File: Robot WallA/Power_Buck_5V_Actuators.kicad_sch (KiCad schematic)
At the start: 18 parts, among them J14 NID35-5, Q1 BSS138

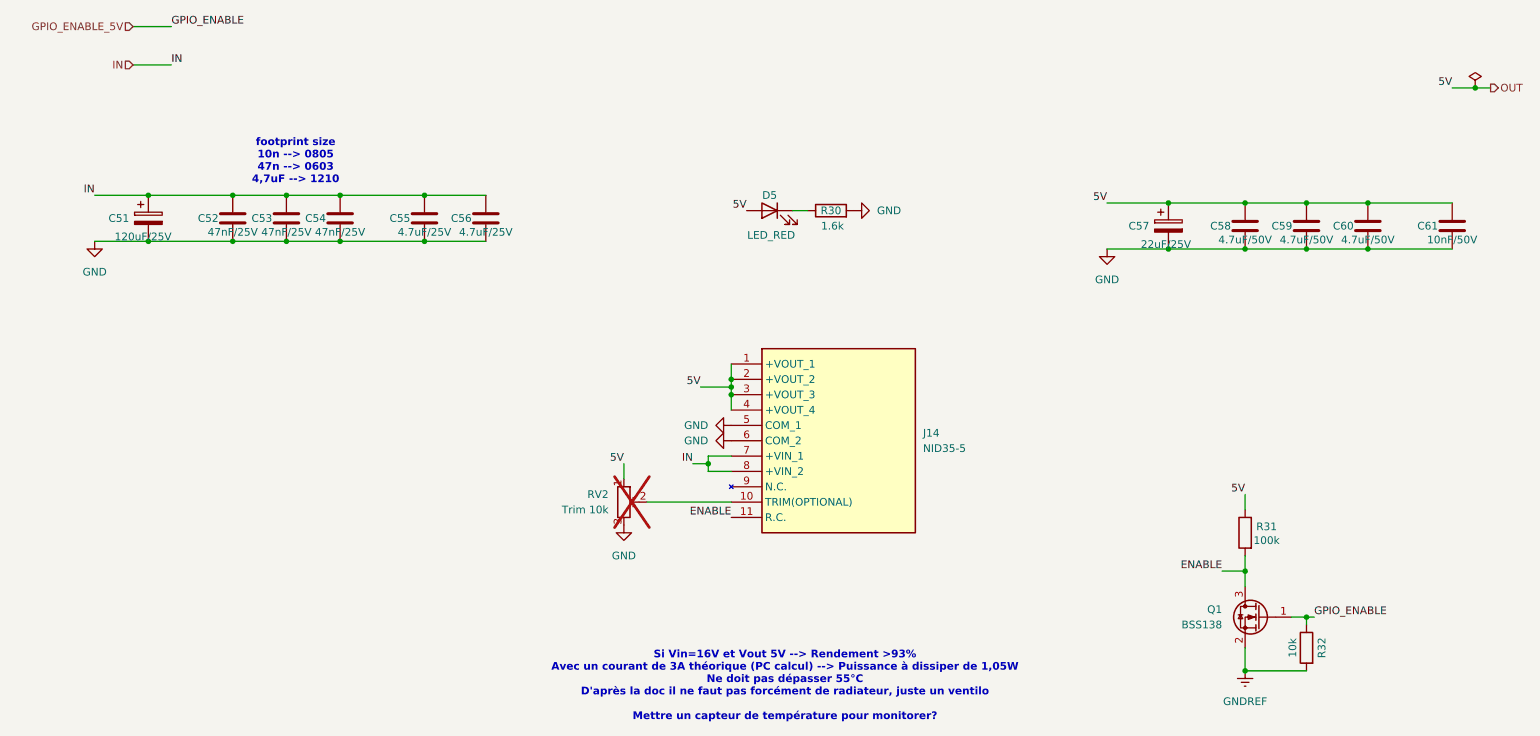
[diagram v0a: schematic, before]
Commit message: Reworked 12V and 5V power supplies, continue routing
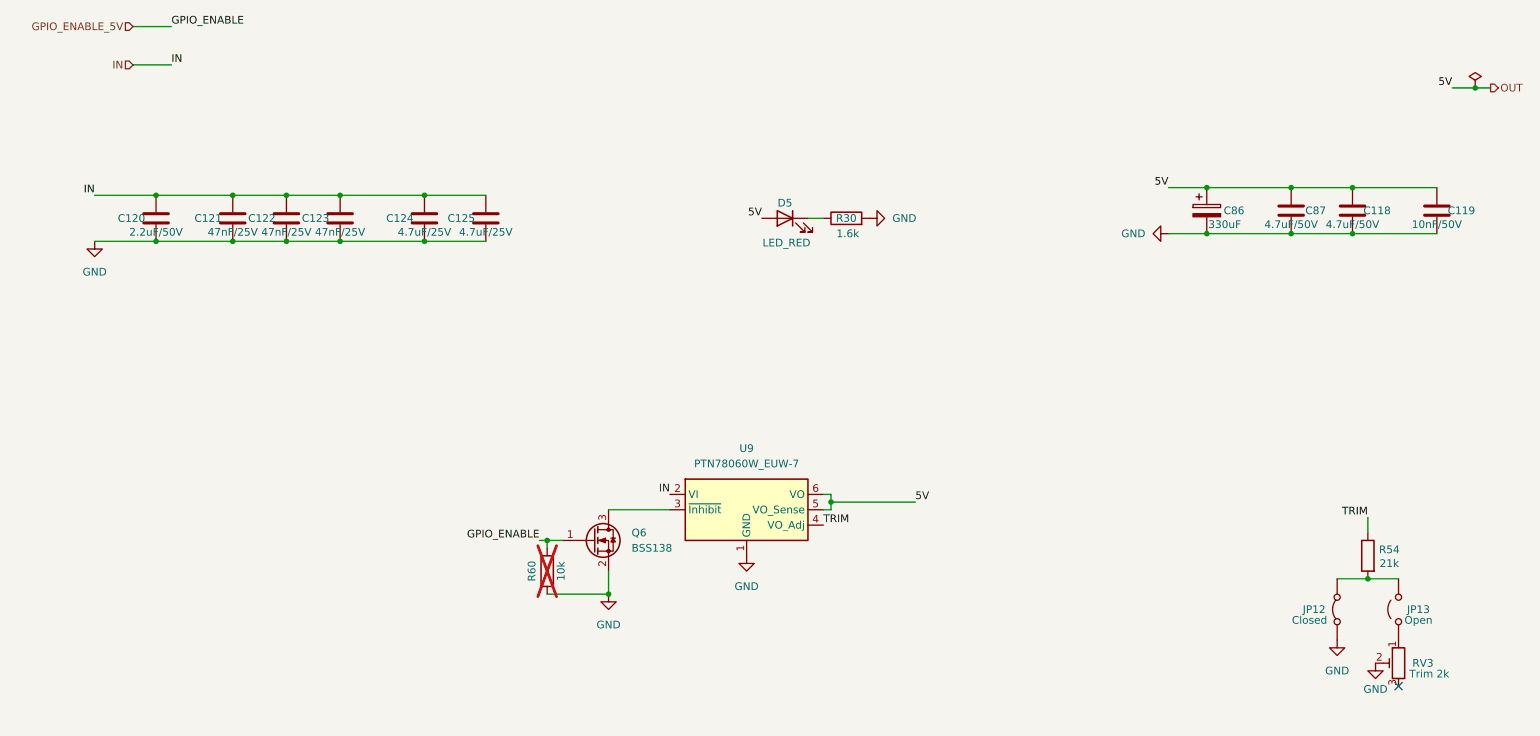
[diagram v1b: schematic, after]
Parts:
- removed C51: 120uF/25V, SamacSys_Parts:EEE0JA331XP, symbol Device:C_Polarized
- removed C52, C53, C54: 47nF/25V, Capacitor_SMD:C_0603_1608Metric_Pad1.08x0.95mm_HandSolder, symbol Device:C
- removed C55, C56: 4.7uF/25V, Capacitor_SMD:C_1210_3225Metric_Pad1.33x2.70mm_HandSolder, symbol Device:C
- removed C57: 22uF/25V, SamacSys_Parts:EEE1AA220WR, symbol Device:C_Polarized
- removed C58, C59, C60: 4.7uF/50V, Capacitor_SMD:C_0805_2012Metric_Pad1.18x1.45mm_HandSolder, symbol Device:C
- removed C61: 10nF/50V, Capacitor_SMD:C_0805_2012Metric_Pad1.18x1.45mm_HandSolder, symbol Device:C
- removed J14: NID35-5, SamacSys_Parts:NID355, symbol SamacSys_Parts:NID35-5
- removed Q1: BSS138, Package_TO_SOT_SMD:SOT-23, symbol Transistor_FET:BSS138
- removed R31: 100k, Resistor_SMD:R_0603_1608Metric_Pad0.98x0.95mm_HandSolder, symbol Device:R
- removed R32: 10k, Resistor_SMD:R_0603_1608Metric_Pad0.98x0.95mm_HandSolder, symbol Device:R
- removed RV2: Trim 10k, SamacSys_Parts:TC33X2503E, symbol Device:R_Potentiometer_Trim
- added C118, C87: 4.7uF/50V, Capacitor_SMD:C_1210_3225Metric_Pad1.33x2.70mm_HandSolder, symbol Device:C
- added C119: 10nF/50V, Capacitor_SMD:C_0805_2012Metric_Pad1.18x1.45mm_HandSolder, symbol Device:C
- added C120: 2.2uF/50V, Capacitor_SMD:C_1210_3225Metric_Pad1.33x2.70mm_HandSolder, symbol Device:C
- added C121, C122, C123: 47nF/25V, Capacitor_SMD:C_0603_1608Metric_Pad1.08x0.95mm_HandSolder, symbol Device:C
- added C124, C125: 4.7uF/25V, Capacitor_SMD:C_1210_3225Metric_Pad1.33x2.70mm_HandSolder, symbol Device:C
- added C86: 330uF, SamacSys_Parts:CAPPRD500W65D1000H1800, symbol Device:C_Polarized
- added JP12: Closed, Jumper:SolderJumper-2_P1.3mm_Bridged_RoundedPad1.0x1.5mm, symbol Jumper:Jumper_2_Bridged
- added JP13: Open, Jumper:SolderJumper-2_P1.3mm_Open_RoundedPad1.0x1.5mm, symbol Jumper:Jumper_2_Open
- added Q6: BSS138, Package_TO_SOT_SMD:SOT-23, symbol Transistor_FET:BSS138
- added R54: 21k, Resistor_SMD:R_0603_1608Metric_Pad0.98x0.95mm_HandSolder, symbol Device:R
- added R60: 10k, Resistor_SMD:R_0603_1608Metric_Pad0.98x0.95mm_HandSolder, symbol Device:R
- added RV3: Trim 2k, SamacSys_Parts:TC42X2202E, symbol Device:R_Potentiometer_Trim
- added U9: PTN78060W_EUW-7, Module:Texas_EUW_R-PDSS-T7_THT, symbol Converter_DCDC:PTN78060W_EUW-7
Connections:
- net GND: now also C118.2, C119.2, C120.2, C121.2, C122.2, C123.2, C124.2, C125.2, C86.2, C87.2, JP12.1 (A), Q6.2 (S), R60.2, RV3.2, U9.1 (GND), U9.7 (GND)
- net GPIO_ENABLE_5V: now also Q6.1 (G), R60.1
- net IN: now also C120.1, C121.1, C122.1, C123.1, C124.1, C125.1, U9.2 (VI)
- net OUT: now also C118.1, C119.1, C86.1, C87.1, U9.5 (VO_Sense), U9.6 (VO)
- new net: Q6.3 (D), U9.3 (~{Inhibit})
- new net: JP12.2 (B), JP13.1 (A), R54.2
- new net: JP13.2 (B), RV3.1
- new net TRIM: R54.1, U9.4 (VO_Adj)
- no-connect marks 0 -> 1
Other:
- note removed: "Si Vin=16V et Vout 5V --> Rendement >93% Avec un courant de 3A théorique (PC calcul) --> Puissance à dissiper de 1,05W Ne doit pas dépasser 55°C D'après la doc il ne faut pas forcément de radiateur, juste un ventilo Mettre un capteur de température pour monitorer?"
- note removed: "footprint size 10n --> 0805 47n --> 0603 4,7uF --> 1210"
- moved on the sheet: D5, R30
